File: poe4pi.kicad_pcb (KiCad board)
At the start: 4 copper layers, 65 x 56 mm, 31 parts, among them J1 Conn_02x02_Odd_Even, J2 Conn_02x02_Odd_Even, J3 Conn_02x20_Odd_Even, U1 LTC4413EDD-2-PBF, U3 TPS2375-1

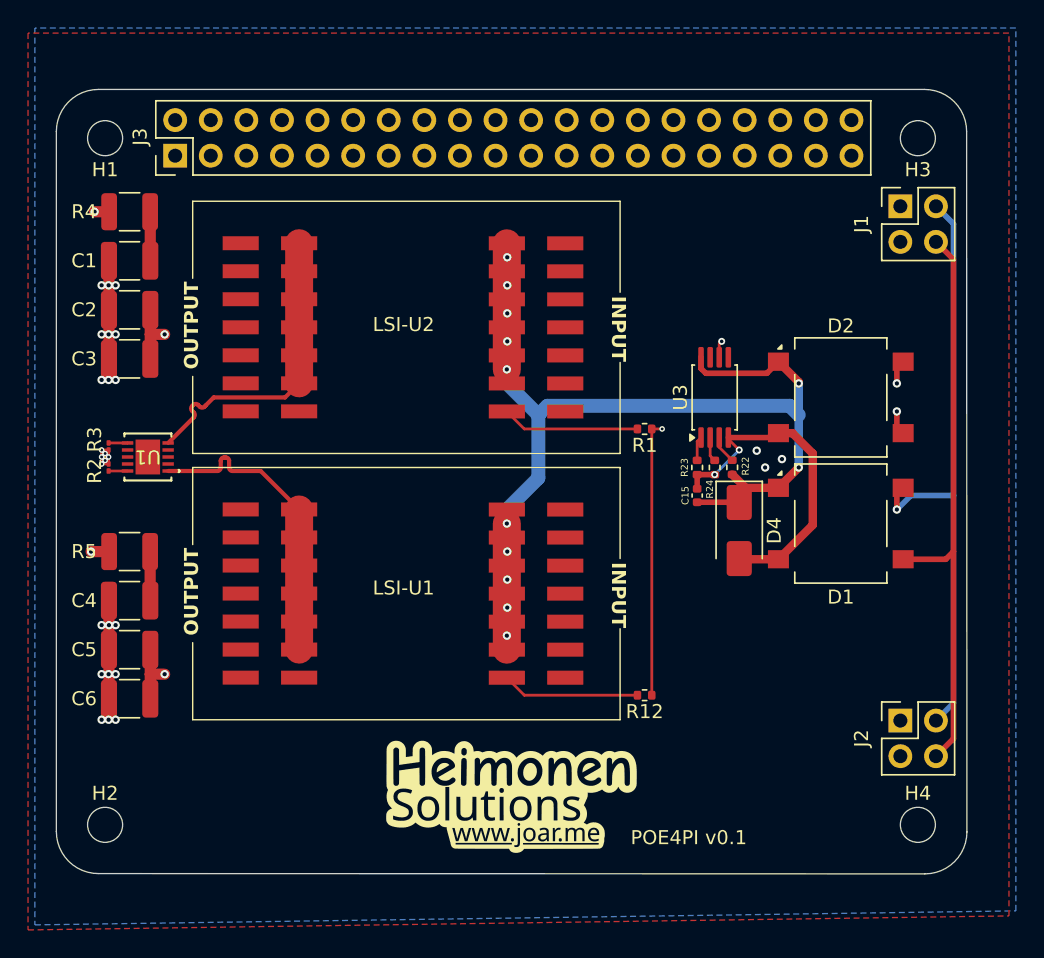
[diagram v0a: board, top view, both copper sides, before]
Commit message: fix: vias
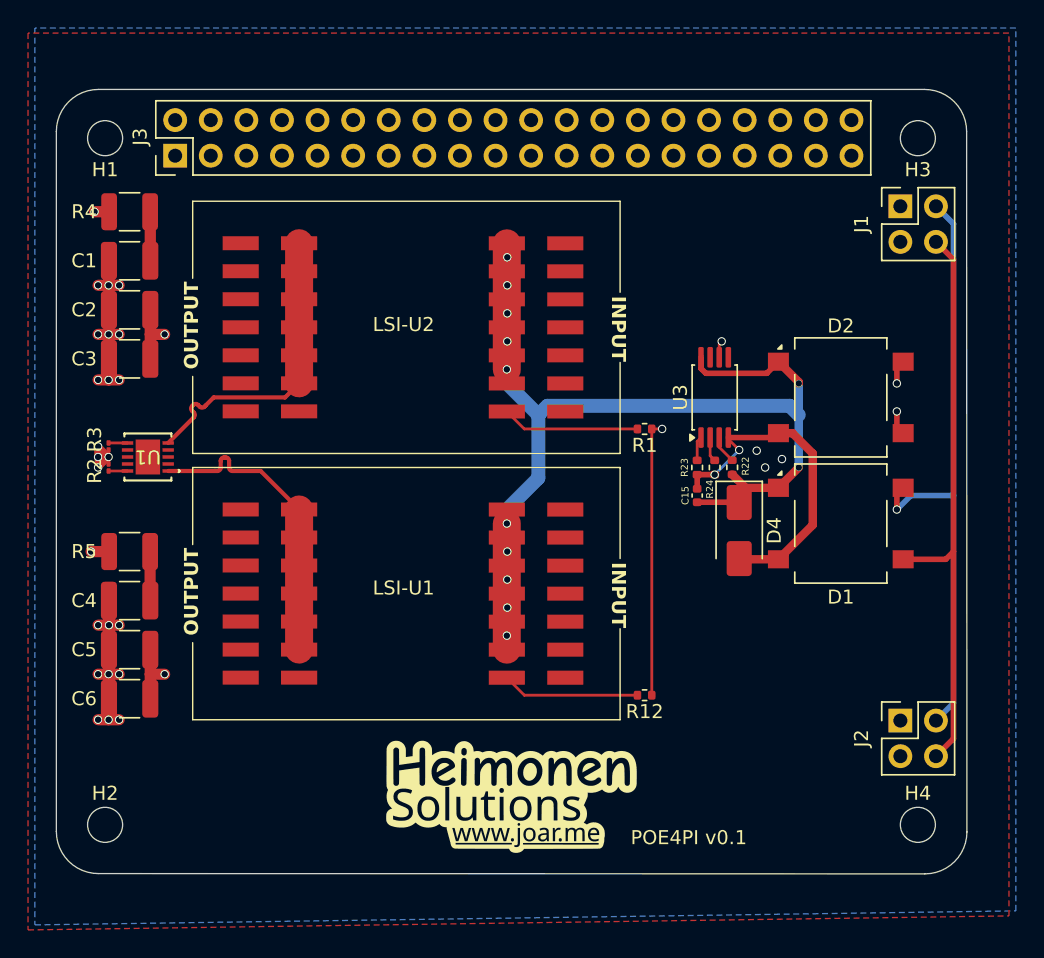
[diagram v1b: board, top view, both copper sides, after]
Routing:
- net +5V: track 18.9 -> 29.1 mm, vias 24 -> 22
